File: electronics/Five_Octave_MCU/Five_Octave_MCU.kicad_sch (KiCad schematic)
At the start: 33 parts, among them J1 FFC Connector, J1 HRO_TYPE-C-31-M-12, SW21 Alps_Alpine_SKRP, SW22 Alps_Alpine_SKRP, U1 AP2112K-3.3, U2 Raspberry_Pi_RP2040, U3 W25Q64JVXGIQ, Y1 12MHz

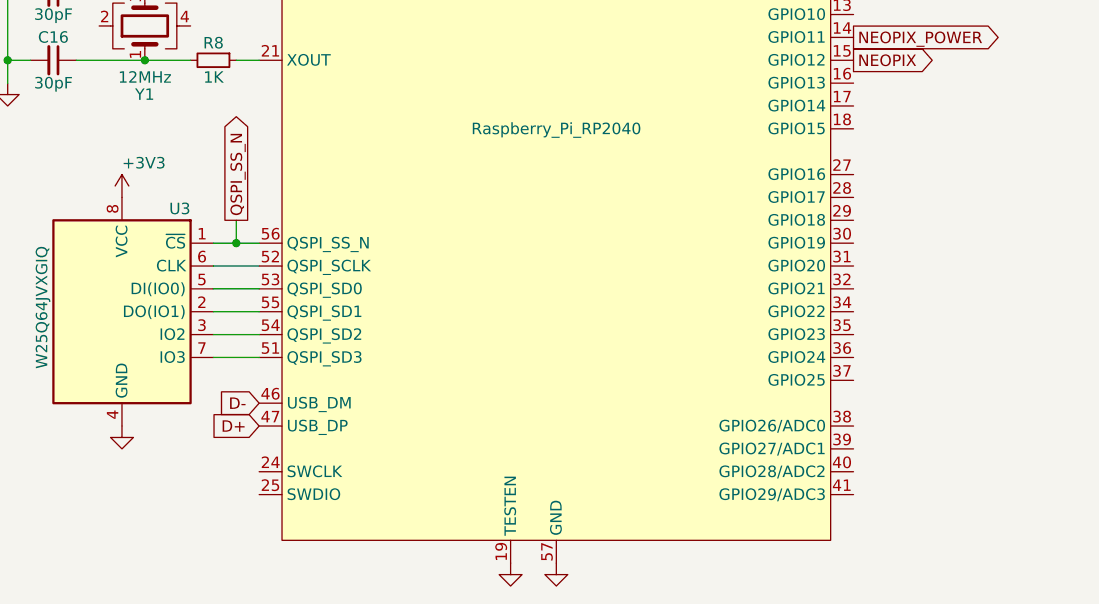
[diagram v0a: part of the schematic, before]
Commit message: WIP
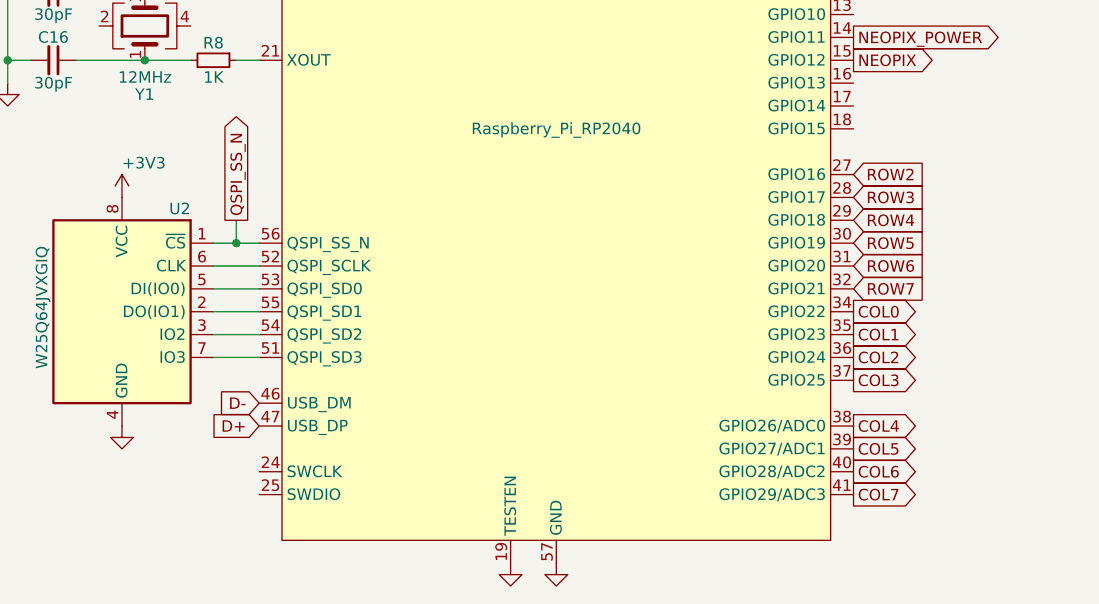
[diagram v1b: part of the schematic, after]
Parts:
- J1: LCSC (none) -> C165948
- LED1: LCSC (none) -> C2976072
- SW21, SW22: LCSC (none) -> C470426
- U1: LCSC (none) -> C51118
- U2: LCSC (none) -> C2040
- U2: renamed from U3; LCSC (none) -> C2940195
- Y1: LCSC (none) -> C9002
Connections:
- net COL0: now also U2.34 (GPIO22)
- net COL1: now also U2.35 (GPIO23)
- net COL2: now also U2.36 (GPIO24)
- net COL3: now also U2.37 (GPIO25)
- net COL4: now also U2.38 (GPIO26/ADC0)
- net COL5: now also U2.39 (GPIO27/ADC1)
- net COL6: now also U2.40 (GPIO28/ADC2)
- net COL7: now also U2.41 (GPIO29/ADC3)
- net ROW2: now also U2.27 (GPIO16)
- net ROW3: now also U2.28 (GPIO17)
- net ROW4: now also U2.29 (GPIO18)
- net ROW5: now also U2.30 (GPIO19)
- net ROW6: now also U2.31 (GPIO20)
- net ROW7: now also U2.32 (GPIO21)

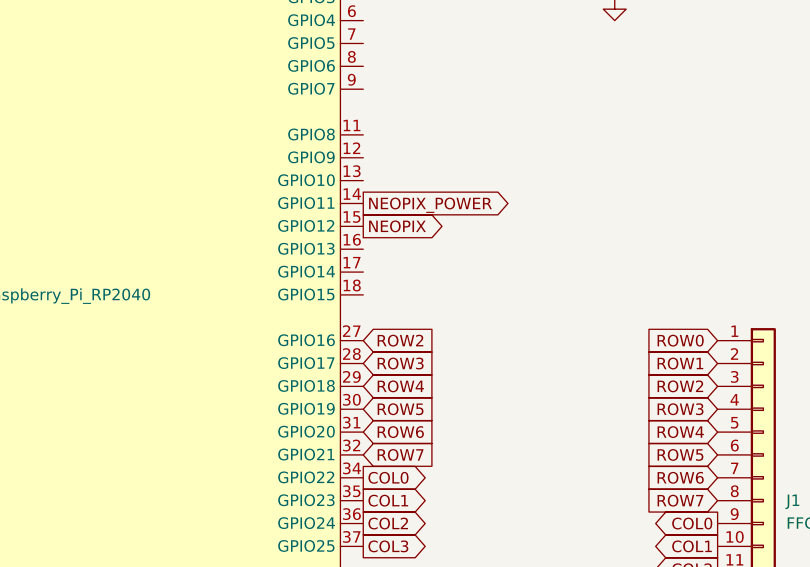
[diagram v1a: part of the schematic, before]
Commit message: WIP
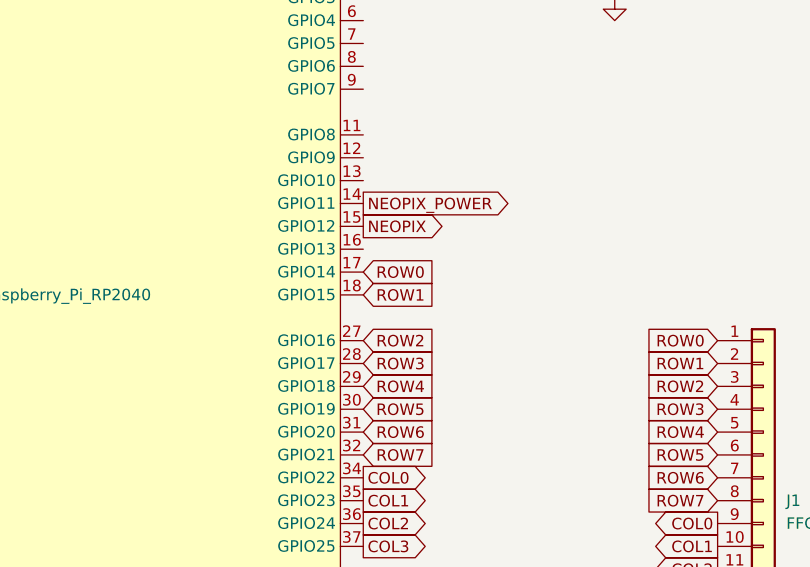
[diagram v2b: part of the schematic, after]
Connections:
- net ROW0: now also U2.17 (GPIO14)
- net ROW1: now also U2.18 (GPIO15)
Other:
- title: (none) -> Five Octave - MCU
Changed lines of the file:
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@@
 (kicad_sch (version 20230121) (generator eeschema)
   (paper "A4")
+  (title_block
+    (title "Five Octave - MCU")
+    (date "2023-08-14")
+    (rev "0.1.0-wip.1")
+    (comment 1 "https://github.com/takayoshiotake/five-octave-61-key-keyboard")
+  )
   (junction (at 133.985 57.785) (diameter 0) (color 0 0 0 0)
   )
@@
     )
   )
+  (global_label "ROW0" (shape input) (at 161.925 106.045 0) (fields_autoplaced)
+    (effects (font (size 1.27 1.27)) (justify left))
+    (property "Intersheetrefs" "${INTERSHEET_REFS}" (at 170.1716 106.045 0)
+      (effects (font (size 1.27 1.27)) (justify left) hide)
+    )
+  )
+  (global_label "ROW1" (shape input) (at 161.925 108.585 0) (fields_autoplaced)
+    (effects (font (size 1.27 1.27)) (justify left))
+    (property "Intersheetrefs" "${INTERSHEET_REFS}" (at 170.1716 108.585 0)
+      (effects (font (size 1.27 1.27)) (justify left) hide)
+    )
+  )
